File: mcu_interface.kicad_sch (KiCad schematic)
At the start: 6 parts, among them U2 MSP430FR2355TPT, Y1 32768

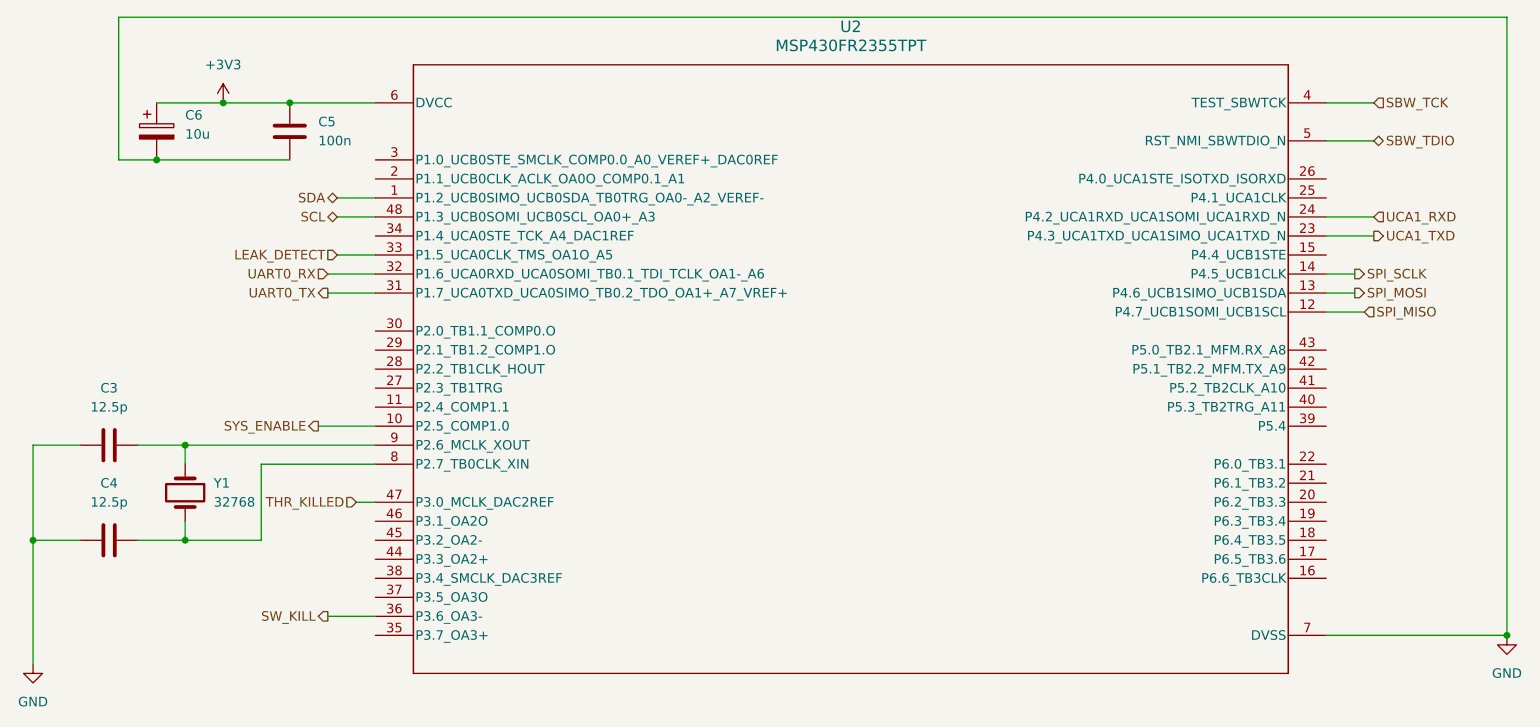
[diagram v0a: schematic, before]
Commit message: Fix a variety of small issues
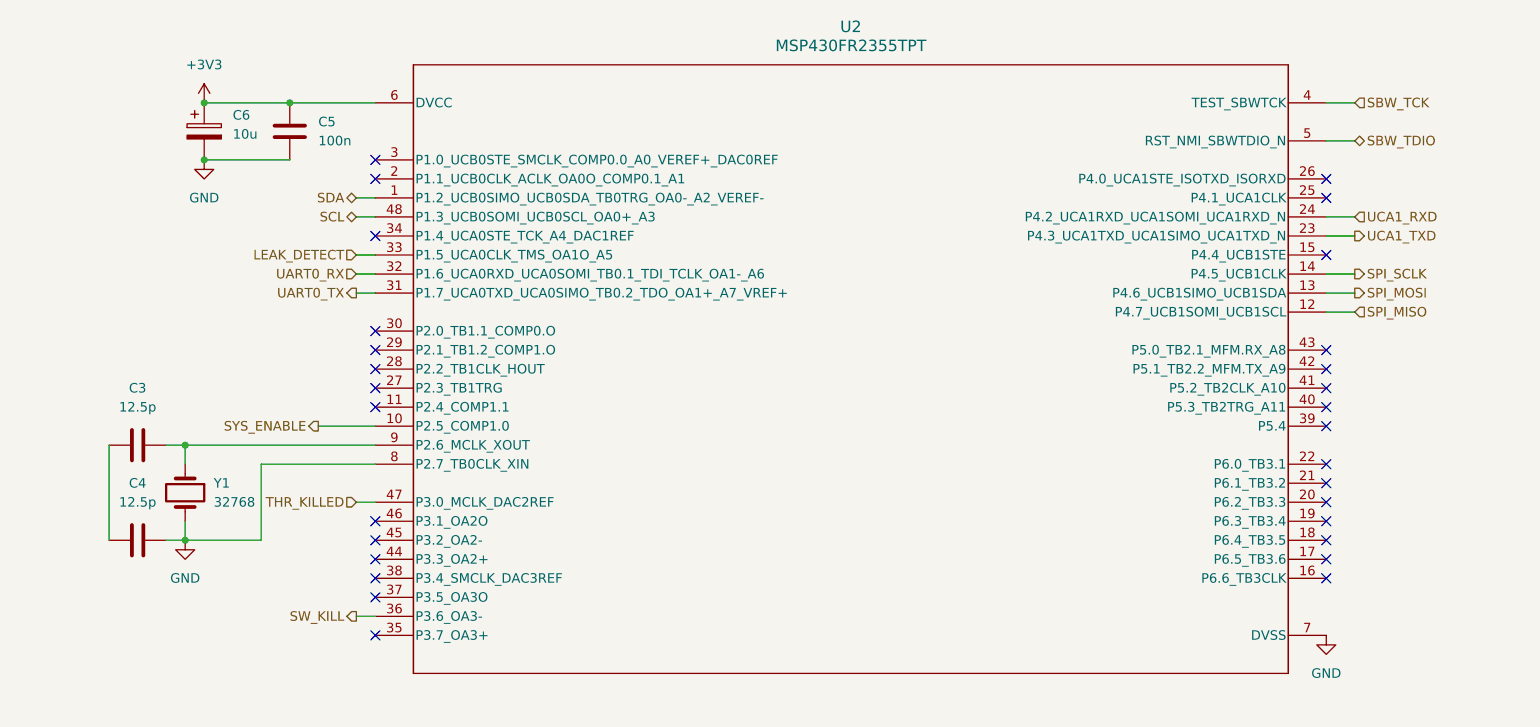
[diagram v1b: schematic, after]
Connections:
- net GND: now also C4.1, U2.8 (P2.7_TB0CLK_XIN), Y1.2; no longer C3.2, C4.2
- new net: C3.2, C4.2
- no-connect marks 0 -> 29
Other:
- moved on the sheet: C3, C4, C6
